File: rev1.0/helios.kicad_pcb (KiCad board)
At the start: 4 copper layers, 17.8 x 33 mm, 59 parts, among them J1 USB_C_Receptacle_USB2.0, J2 helios-pinout, Q1 2N7002VC-, Q2 2N7002VC-, SW1 SWITCH, U1 USBLC6-2P6, U2 TLV75533PDQNR, U3 W25Q128JVPIQ, U4 RP2040, U5 74LVC1T45, Y1 12MHz

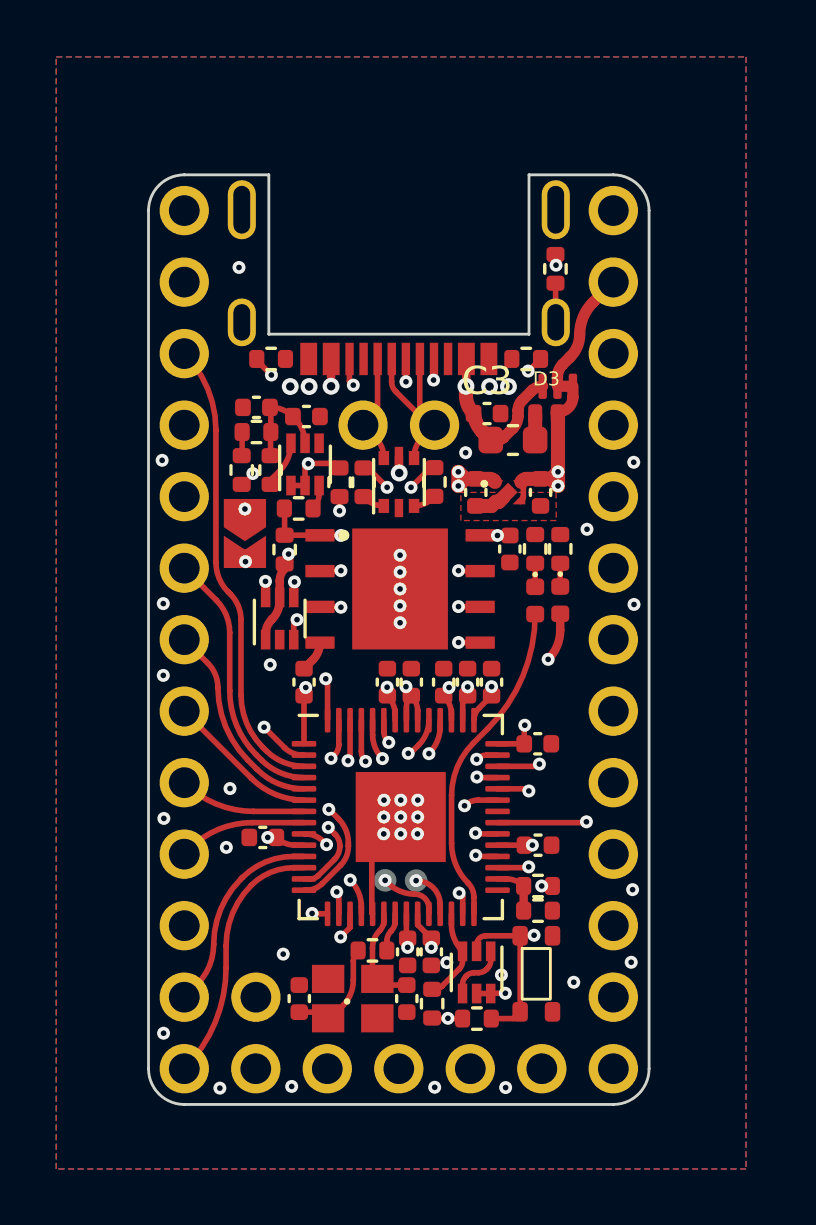
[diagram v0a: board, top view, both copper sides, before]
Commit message: prod files
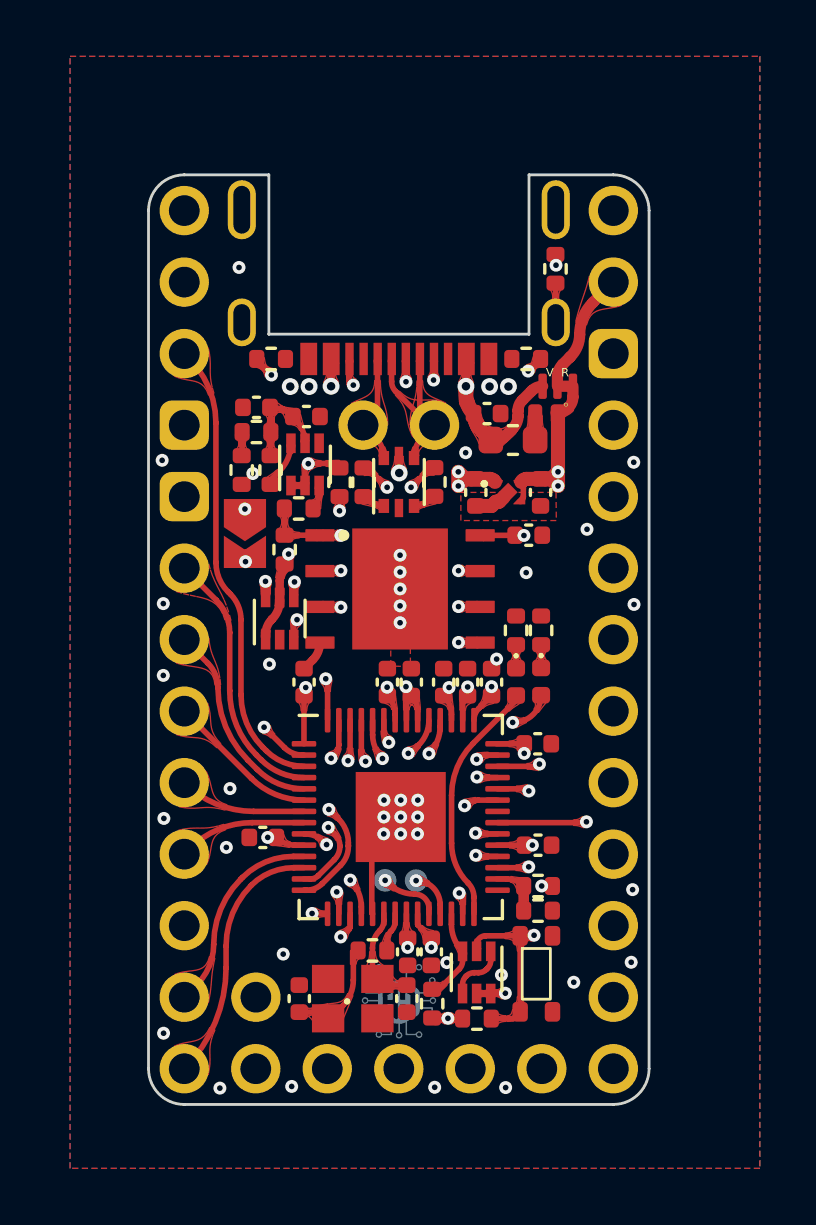
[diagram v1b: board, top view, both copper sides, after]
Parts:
- added REF**: LOGO, art:LOGO, B.Cu at (158.9, 162.2)
- moved D2 2.97 mm to (163.0, 150.9)
- moved D1 2.97 mm to (163.9, 150.9)
- moved R10 2.97 mm to (163.9, 149.1)
- moved R15 2.97 mm to (163.0, 149.1)
- moved C6 0.83 mm to (163.5, 145.7), turned to 0 degrees
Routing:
- net /LED: track 11.7 -> 8.77 mm
- net Net-(D1-Pad2): track 24.1 -> 22.3 mm
- net +3V3: track 20.6 -> 21.3 mm, vias 16 -> 15
- net GND: vias 42 -> 45
